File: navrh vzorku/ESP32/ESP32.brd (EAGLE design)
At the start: 63.5 x 70.8 mm, 20 parts, among them U1 ESP-WROOM-32

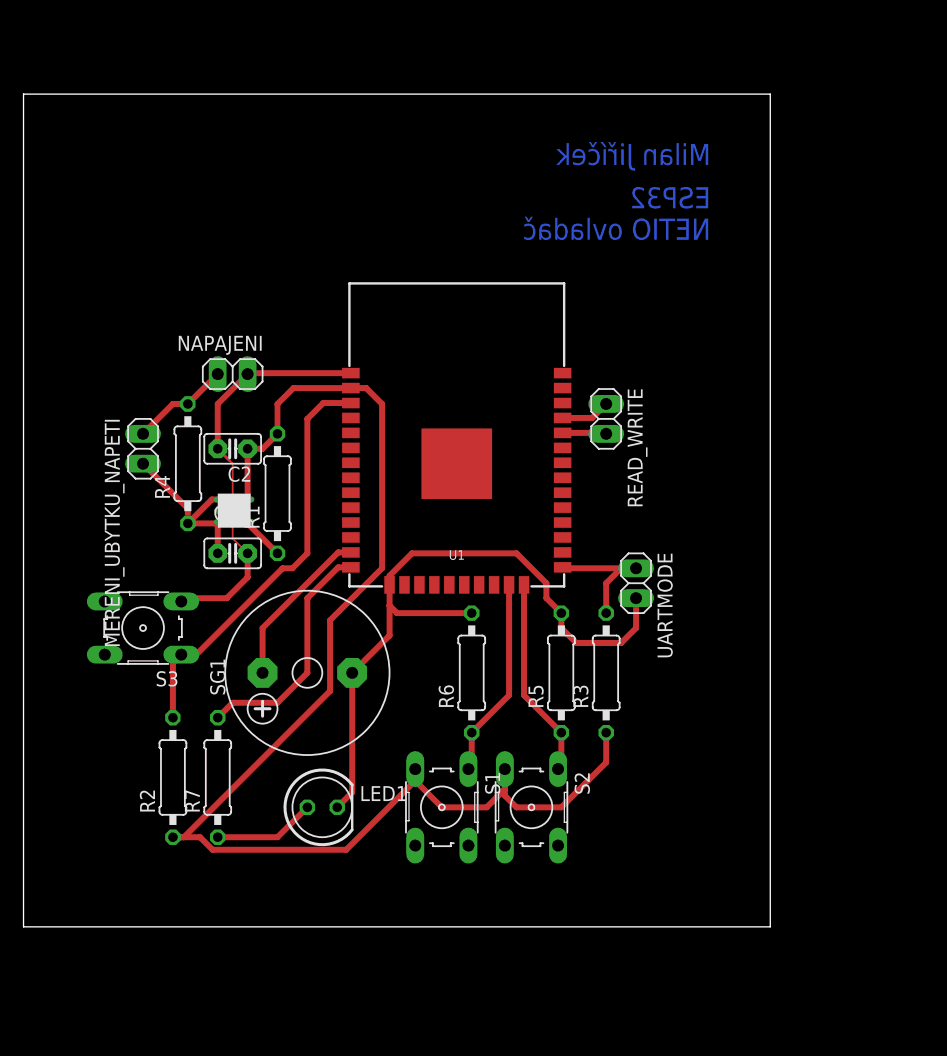
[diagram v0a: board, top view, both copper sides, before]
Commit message: Plosne spoje
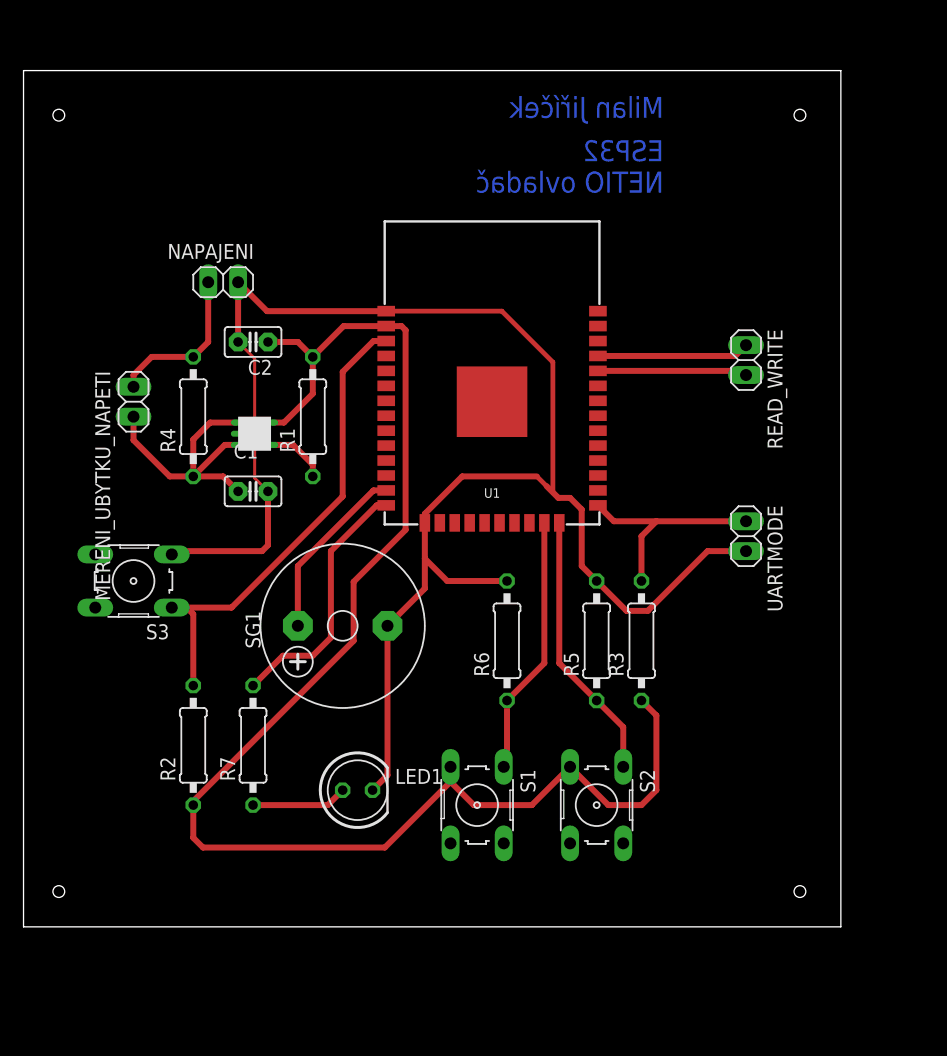
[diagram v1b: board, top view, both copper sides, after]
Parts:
- R7: value 100k -> 10
- moved READ_WRITE 12.9 mm to (61.4, 48.2)
- moved UARTMODE 10.2 mm to (61.4, 33.2)
- moved C2 9.24 mm to (19.5, 49.7)
- moved NAPAJENI 7.85 mm to (17.0, 54.8)
- moved R1 7.20 mm to (24.6, 43.4)
- moved U$1 6.76 mm to (18.2, 43.4)
- moved U1 6.06 mm to (39.8, 44.6)
- moved C1 5.55 mm to (19.5, 37.0)
- moved S2 5.54 mm to (48.7, 10.3)
- moved SG1 5.00 mm to (27.1, 25.6)
- moved MERENI_UBYTKU_NAPETI 4.08 mm to (9.35, 44.6)
- moved S3 4.08 mm to (9.35, 29.4)
- moved R3 4.06 mm to (52.5, 24.3)
- moved R5 4.06 mm to (48.7, 24.3)
- moved R6 4.06 mm to (41.1, 24.3)
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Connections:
- removed net N$16: LED1.K, R5.2, R6.2, SG1.-, U1.15, UARTMODE.2
- removed net N$3: C1.2, C2.2, NAPAJENI.1, S3.3, U$1.GND, U1.1
- new net GND: C1.2, C2.2, LED1.K, NAPAJENI.1, R5.2, R6.2, S3.3, S3.4, SG1.-, U$1.GND, U1.1, U1.15, UARTMODE.2
- net N$5: now also S3.2
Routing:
- net GND: track 0.00 -> 146.3 mm
- net N$16: track 58.2 -> 0.00 mm
- net N$3: track 35.8 -> 0.00 mm
- net N$2: track 115.5 -> 127.2 mm
- net N$1: track 15.8 -> 25.0 mm
- net N$6: track 3.73 -> 12.7 mm
- net N$7: track 4.19 -> 13.0 mm
- net N$8: track 10.6 -> 18.8 mm
- net N$5: track 35.6 -> 42.0 mm
- net N$11: track 17.1 -> 23.0 mm
- net N$10: track 8.45 -> 13.6 mm
- net N$12: track 17.1 -> 22.2 mm
- net N$9: track 20.3 -> 22.0 mm
- net N$4: track 3.71 -> 5.15 mm
- net N$13: track 14.0 -> 15.3 mm
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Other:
- board size 63.5 x 70.8 mm -> 69.5 x 72.8 mm

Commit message: Finalni verze
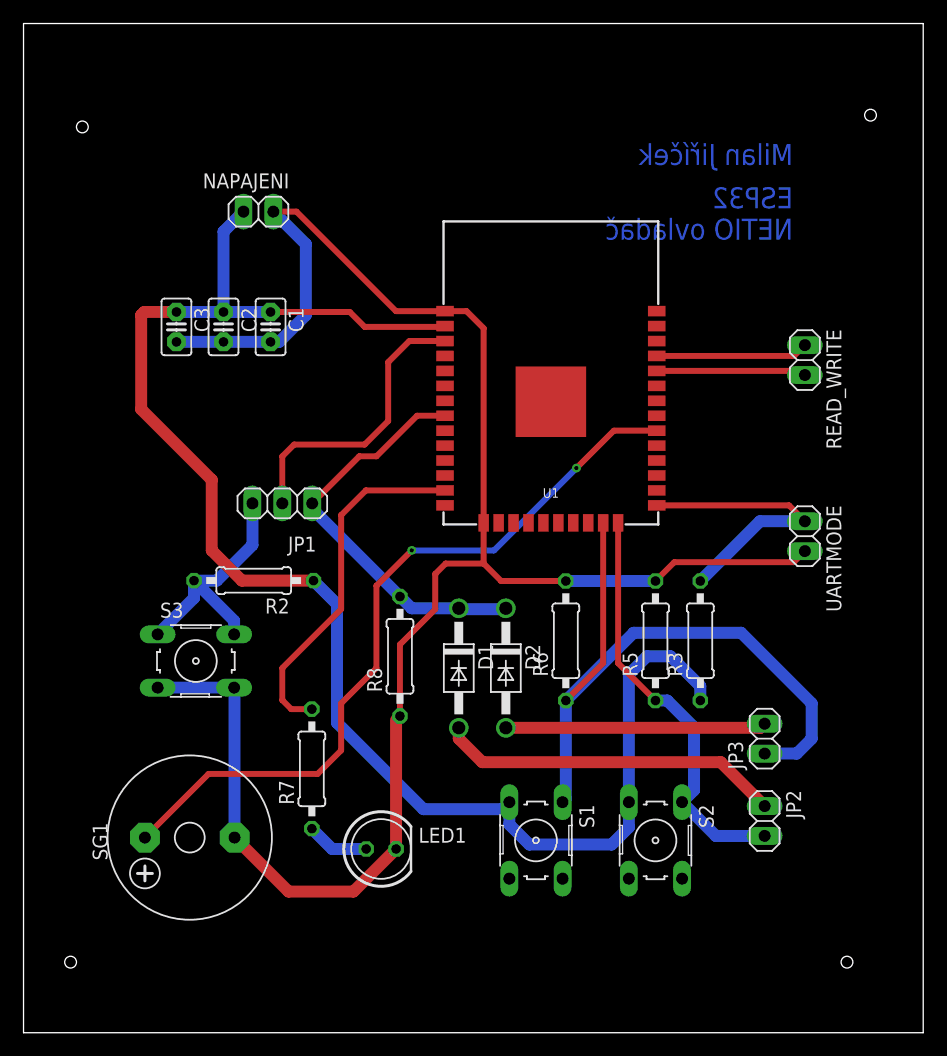
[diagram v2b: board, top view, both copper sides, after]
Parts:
- removed MERENI_UBYTKU_NAPETI: (no value), pinhead:1X02
- removed R1: 100k, rcl:0207/10
- removed R4: 10, rcl:0207/10
- removed U$1: LDLN030, WT8266:LDLN030
- added C3: 0.1u, capacitor-wima:C2.5-2
- added D1, D2: 1N4004, diode:DO41-10
- added JP1: (no value), pinhead:1X03
- added JP2, JP3: (no value), pinhead:1X02
- added R8: (no value), rcl:0207/10
- C1, C2: value (none) -> 22u
- moved SG1 22.2 mm to (14.1, 7.59)
- moved R2 14.9 mm to (19.6, 29.4), turned to 180 degrees
- moved C1 14.1 mm to (21.0, 51.0), turned to 270 degrees
- moved S3 8.62 mm to (14.7, 22.6), turned to 0 degrees
- moved NAPAJENI 6.71 mm to (20.0, 60.8)
- moved S1 5.83 mm to (43.6, 7.35)
- moved S2 5.83 mm to (53.7, 7.35)
- moved R7 5.39 mm to (24.5, 13.4)
- moved LED1 5.39 mm to (30.4, 6.62)
- moved R3 5.00 mm to (57.5, 24.3)
- moved R5 5.00 mm to (53.7, 24.3)
- moved R6 5.00 mm to (46.1, 24.3)
- moved READ_WRITE 5.00 mm to (66.4, 48.2)
- moved U1 5.00 mm to (44.8, 44.6)
- moved UARTMODE 5.00 mm to (66.4, 33.2)
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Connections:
- removed net N$10: MERENI_UBYTKU_NAPETI.1, NAPAJENI.2, R4.2
- removed net N$4: R1.1, U$1.PG
- removed net N$9: R7.2, U1.14
- new net N$15: D1.C, D2.C, JP1.1, R8.2, U1.8
- new net N$17: D1.A, JP2.1
- new net N$18: D2.A, JP3.2
- new net N$3: JP1.3, R2.2, S3.1, S3.2
- net GND: now also C3.2, R8.1; no longer U$1.GND
- net N$1: now also SG1.+, U1.30; no longer C1.1, MERENI_UBYTKU_NAPETI.2, R4.1, U$1.EN, U$1.IN
- net N$11: now also JP2.2
- net N$12: now also JP3.1
- net N$13: now also R7.2; no longer SG1.+
- net N$2: now also C1.1, C3.1, NAPAJENI.2; no longer R1.2, U$1.OUT
- net N$5: now also JP1.2; no longer R2.2, S3.1, S3.2
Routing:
- net N$1: track 25.0 -> 64.3 mm, vias 0 -> 2
- net N$12: track 22.2 -> 58.5 mm
- net N$15: track 0.00 -> 35.0 mm
- net N$17: track 0.00 -> 29.3 mm
- net N$18: track 0.00 -> 22.1 mm
- net N$9: track 22.0 -> 0.00 mm
- net N$3: track 0.00 -> 21.6 mm
- net N$5: track 42.0 -> 24.8 mm
- net N$13: track 15.3 -> 30.3 mm
- net N$10: track 13.6 -> 0.00 mm
- net N$11: track 23.0 -> 35.6 mm
- net GND: track 146.3 -> 158.8 mm
- net N$2: track 127.2 -> 134.5 mm
- net N$8: track 18.8 -> 24.1 mm
- net N$4: track 5.15 -> 0.00 mm
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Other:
- board size 69.5 x 72.8 mm -> 76.5 x 85.8 mm
